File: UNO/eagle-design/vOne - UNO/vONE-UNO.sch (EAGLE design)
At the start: 24 parts, among them IC1 ATMEGA328-20P, IC2 7805T, IC4 LM1117MP-3.3, Q1 16 MHz

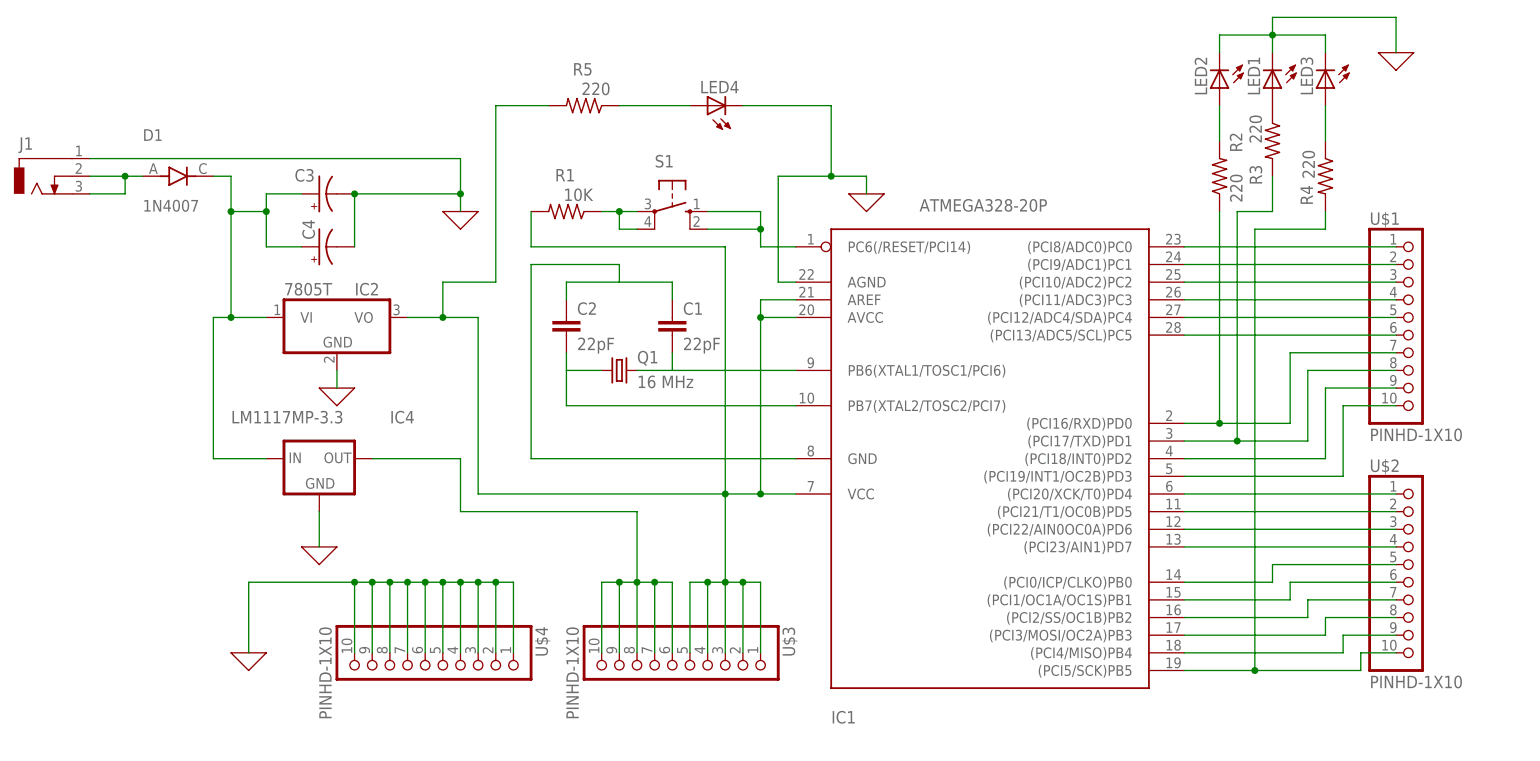
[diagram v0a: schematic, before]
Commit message: Final design complete
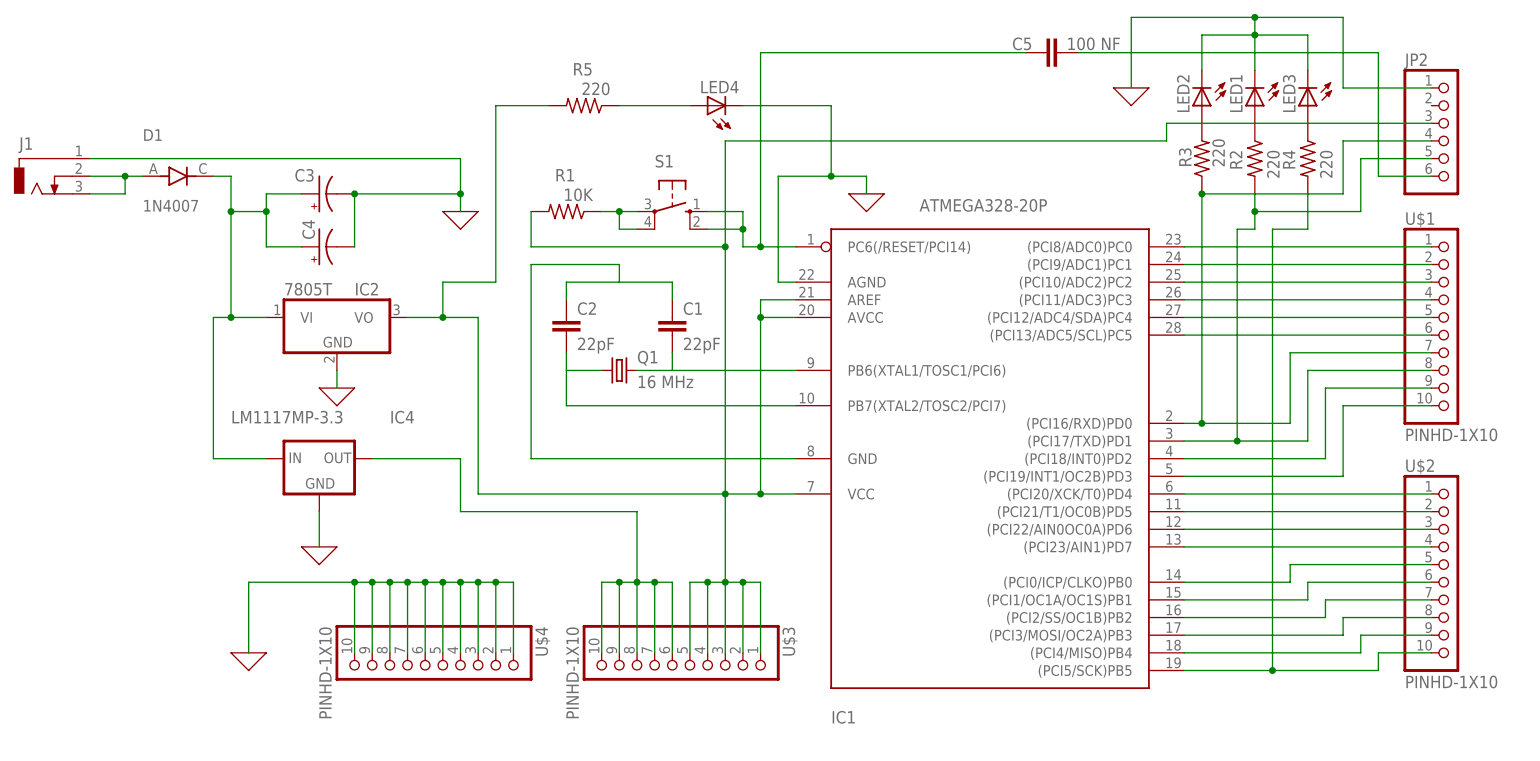
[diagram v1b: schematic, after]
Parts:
- added C5: 100 NF, capacitor-wima:C2,5-3
- added JP2: (no value), adafruit:PINHD-1X6B
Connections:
- new net N$21: C5.2, JP2.6
- net 0: now also JP2.1
- net N$10: now also JP2.4
- net N$2: now also C5.1
- net N$32: now also JP2.3
- net N$37: now also JP2.5
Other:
- moved on the sheet: LED1, LED2, LED3, R2, R3, R4, U$1, U$2
